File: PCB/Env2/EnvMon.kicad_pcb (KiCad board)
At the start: 2 copper layers, 70 x 70 mm, 39 parts, among them J1 LCD, J2 DC, J3 TEMP, J4 LCD, J5 Reset, J6 USB-C-Socket-H, J7 TC2030-USB-NL-DS, J8 T6793, U1 ESP32-S3-MINI-1, U2 SCD41, U3 MD8942, U4 MCP9808_MSOP, U8 VEML6040

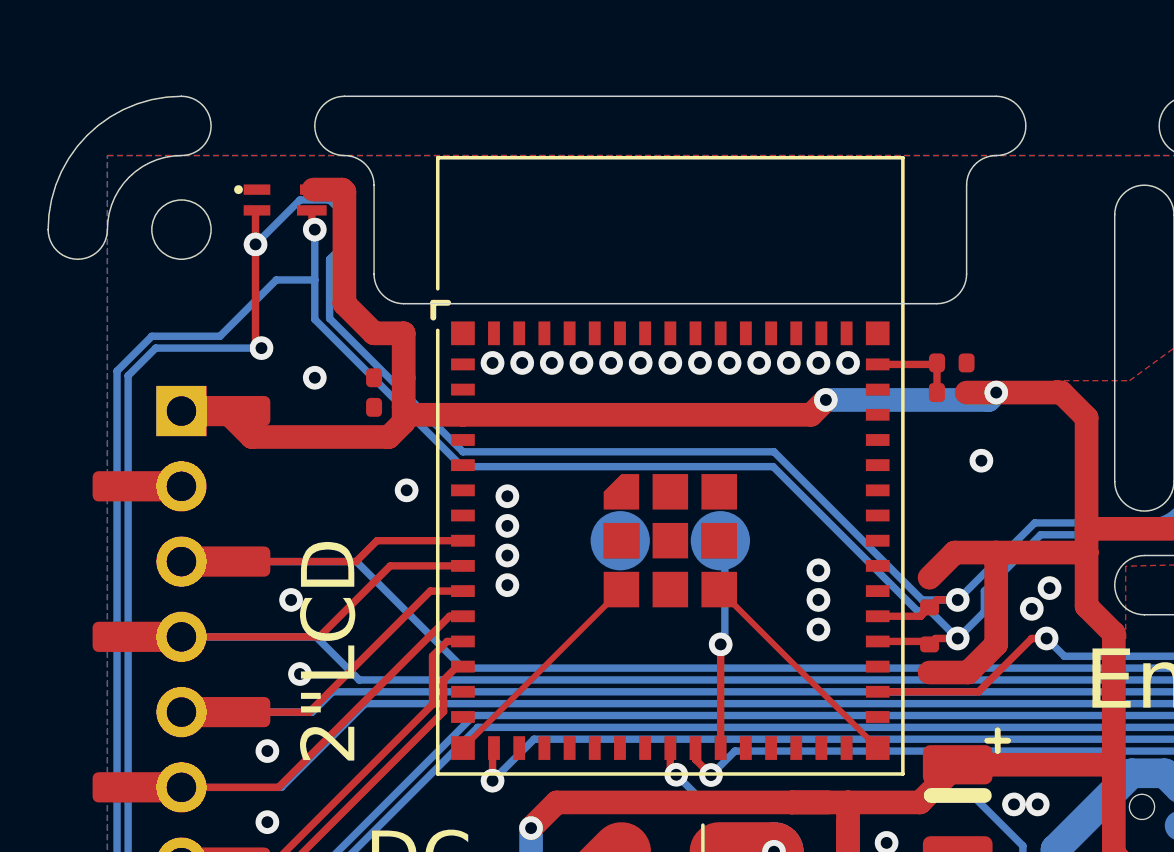
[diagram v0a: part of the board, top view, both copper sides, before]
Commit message: Render
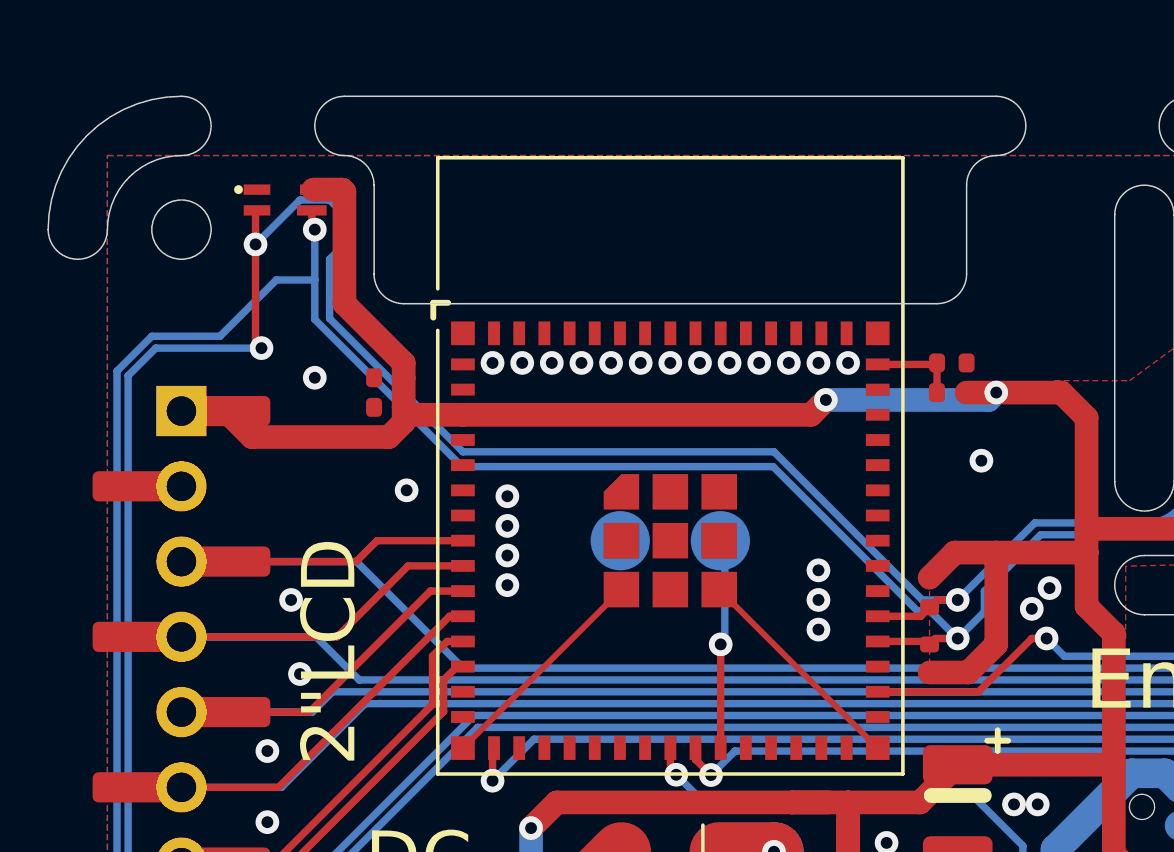
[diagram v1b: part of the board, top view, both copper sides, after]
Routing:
- net +3.3V: track 231.6 -> 231.0 mm
